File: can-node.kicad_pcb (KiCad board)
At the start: 2 copper layers, 116 x 100.2 mm, 41 parts, among them J1 Conn_01x02_Pin, J10 Conn_01x06_Pin, J11 Conn_01x01_Socket, J12 Conn_01x01_Socket, J13 Conn_01x01_Socket, J14 Conn_01x01_Socket, J15 Conn_01x03_Pin, J18 Conn_01x01_Socket, J19 Conn_01x01_Socket, J2 Conn_01x02_Pin, J20 Conn_01x01_Socket, J21 Conn_01x01_Socket, J3 RJ45, J4 RJ45, J5 Conn_01x10_Pin, J6 Conn_01x04_Pin, J7 Conn_01x02_Pin, J8 Conn_01x01_Socket, J9 Conn_01x01_Socket, SW1 SW_DIP_x04, U1 ESP32-DEVKIT-V1

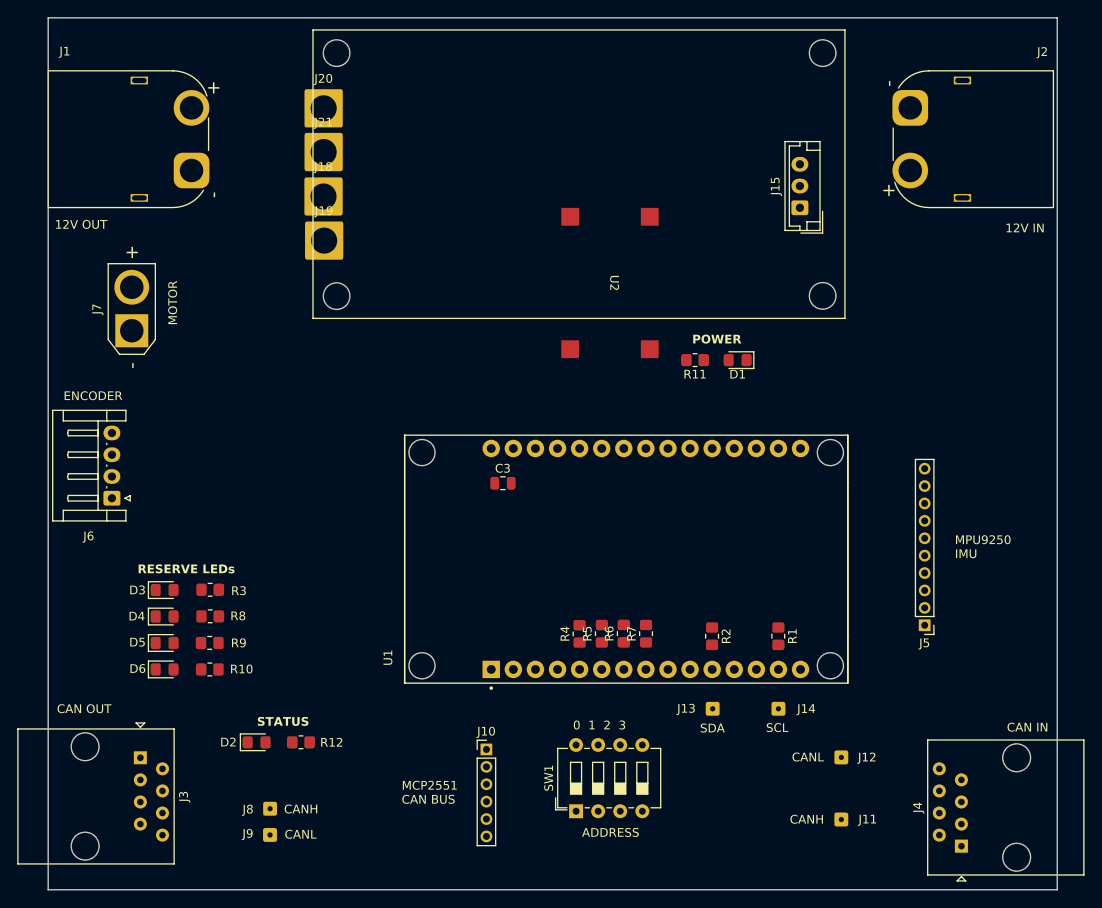
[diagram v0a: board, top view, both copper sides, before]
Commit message: draft?
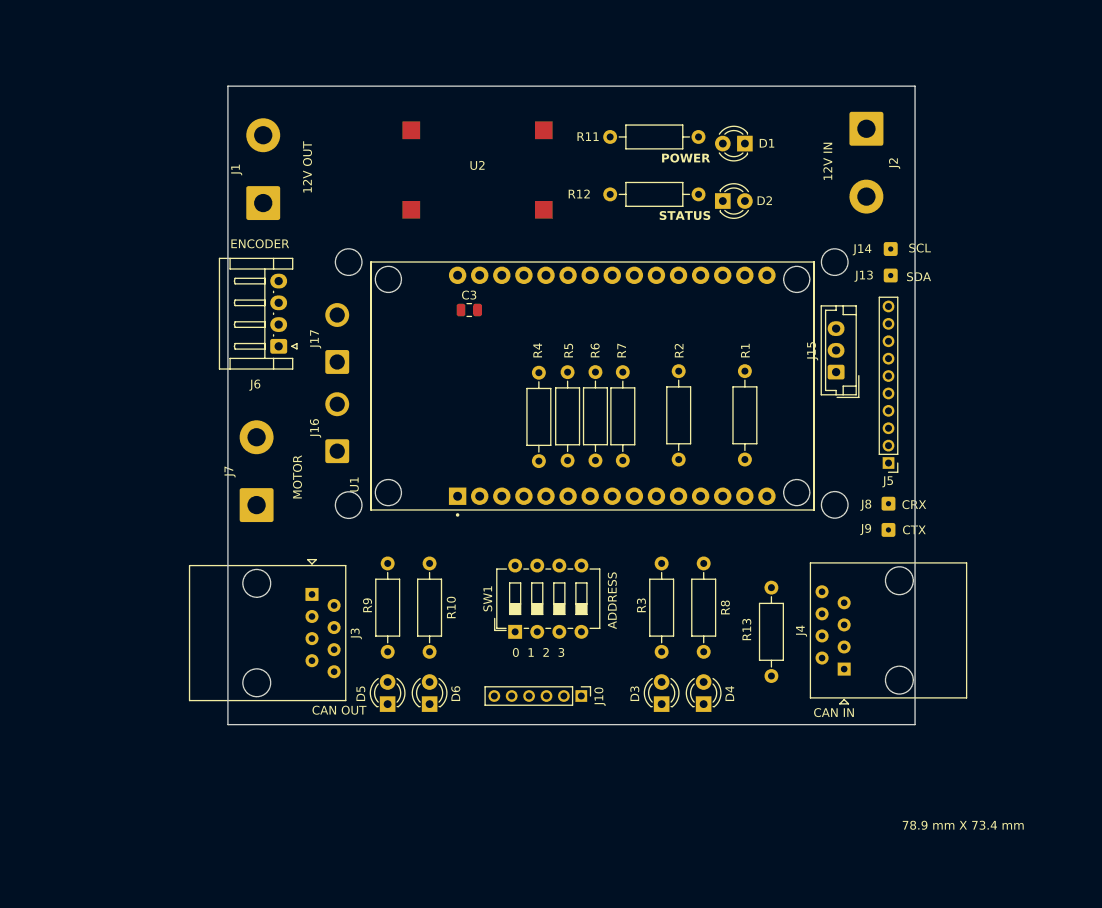
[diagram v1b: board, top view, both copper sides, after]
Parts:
- removed J11, J12: Conn_01x01_Socket, Connector_Wire:SolderWire-0.1sqmm_1x01_D0.4mm_OD1mm
- removed J18, J19, J20, J21: Conn_01x01_Socket, Connector_Wire:SolderWire-2.5sqmm_1x01_D2.4mm_OD4.4mm
- added J16: Conn_01x02_Pin, Connector_Wire:SolderWire-1sqmm_1x02_P5.4mm_D1.4mm_OD2.7mm, F.Cu at (64.1, 73.2)
- added J17: Conn_01x02_Pin, Connector_Wire:SolderWire-1sqmm_1x02_P5.4mm_D1.4mm_OD2.7mm, F.Cu at (64.1, 63.0)
- added R13: 60, Resistor_THT:R_Axial_DIN0207_L6.3mm_D2.5mm_P10.16mm_Horizontal, F.Cu at (114.0, 88.9)
- D1, D2, D3, D4, D5, D6: footprint LED_SMD:LED_0805_2012Metric_Pad1.15x1.40mm_HandSolder -> LED_THT:LED_D3.0mm
- J1, J2: footprint Connector_AMASS:AMASS_XT60PW-M_1x02_P7.20mm_Horizontal -> Connector_Wire:SolderWire-1.5sqmm_1x02_P7.8mm_D1.7mm_OD3.9mm
- J7: footprint Connector_AMASS:AMASS_XT30U-F_1x02_P5.0mm_Vertical -> Connector_Wire:SolderWire-1.5sqmm_1x02_P7.8mm_D1.7mm_OD3.9mm
- R1, R10, R11, R12, R2, R3, R4, R5, R6, R7, R8, R9: footprint Resistor_SMD:R_0805_2012Metric_Pad1.20x1.40mm_HandSolder -> Resistor_THT:R_Axial_DIN0207_L6.3mm_D2.5mm_P10.16mm_Horizontal
- moved D2 82.1 mm to (108.5, 44.5)
- moved J9 79.3 mm to (127.5, 82.3)
- moved J8 79.3 mm to (127.5, 79.2)
- moved R12 72.3 mm to (95.5, 43.7)
- moved D4 62.8 mm to (106.3, 102.3), turned to 90 degrees
- moved D3 58.6 mm to (101.4, 102.3), turned to 90 degrees
- moved R8 56.9 mm to (106.3, 96.3), turned to 90 degrees
- moved J14 54.4 mm to (127.8, 50.0), turned to 180 degrees
- moved J13 53.9 mm to (127.8, 53.0)
- moved R3 52.4 mm to (101.4, 96.3), turned to 90 degrees
- moved D6 30.7 mm to (74.7, 102.3), turned to 90 degrees
- moved R1 30.7 mm to (111.0, 64.0)
- moved R2 30.7 mm to (103.4, 64.0)
- moved J3 27.2 mm to (61.2, 89.7)
- moved D5 26.6 mm to (69.9, 102.3), turned to 90 degrees
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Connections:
- J8 pad 1: CAN+ -> CAN-Rx
- J9 pad 1: CAN- -> CAN-Tx
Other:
- board size 116 x 100.2 mm -> 79 x 73.4 mm
- board text added: "78.9 mm X 73.4 mm"
- board text added: "CRX"
- board text added: "CTX"
- board text removed: "CANH"
- board text removed: "CANL"
- board text removed: "MCP2551 CAN BUS"
- board text removed: "MPU9250 IMU"
- board text removed: "RESERVE LEDs"
